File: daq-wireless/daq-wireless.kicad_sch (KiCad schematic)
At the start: 34 parts, among them J1 5223004-2, J2 Micro_SD_Card, J3 USB_C_Receptacle_USB2.0, Q1 MMBT3904, Q2 MMBT3904, SW1 RESET, U1 ESP32-WROOM-32, U2 AMS1117, U3 FT231XS, U5 Ebyte_E01-ML01SP4

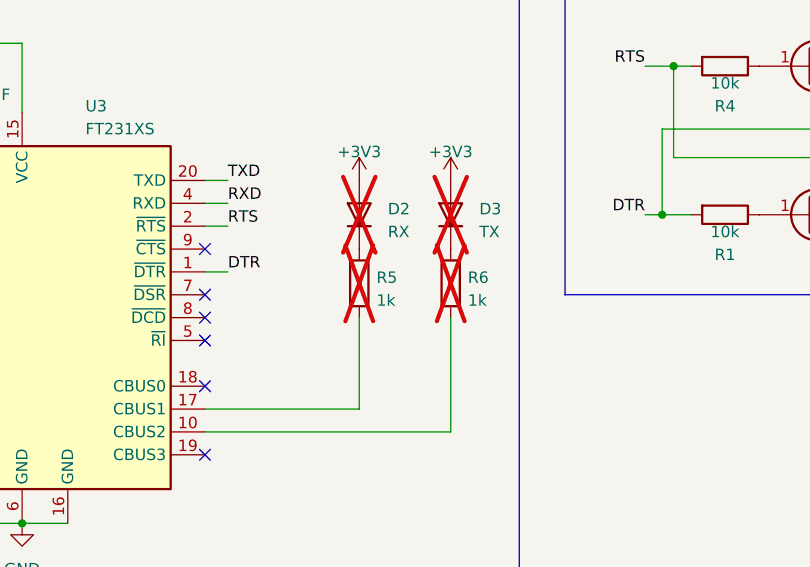
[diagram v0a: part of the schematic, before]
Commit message: BOM
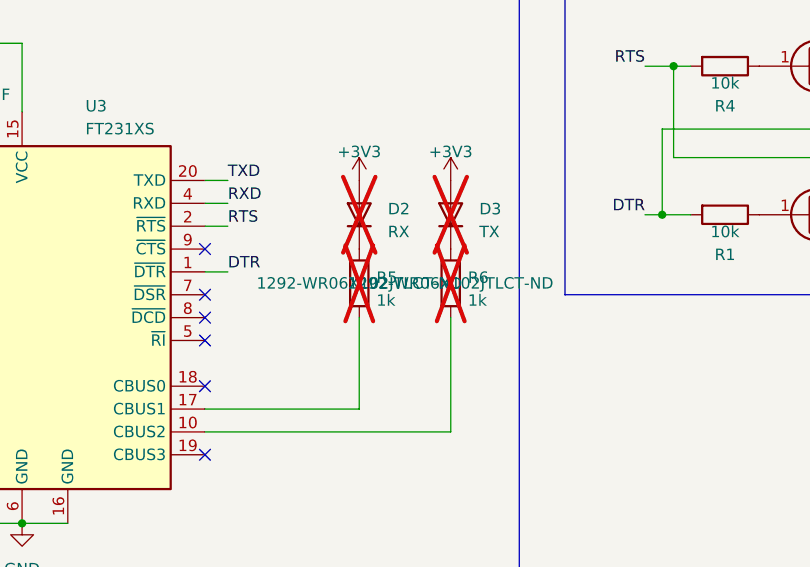
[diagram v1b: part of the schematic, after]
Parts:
- C1, C10, C3, C7, C9: DPN (none) -> 1276-1043-1-ND
- C10: footprint Capacitor_SMD:C_0402_1005Metric -> Capacitor_SMD:C_0603_1608Metric; DPN (none) -> 1276-1102-1-ND
- C2, C6, C8: DPN (none) -> 1276-1102-1-ND
- C4, C5: DPN (none) -> 1276-6460-1-ND
- C8: DPN (none) -> 1276-1119-1-ND
- R1, R4, R7, R8, R9: DPN (none) -> 1292-WR06X103JTLCT-ND
- R2, R3: DPN (none) -> RMCF0603JT5K10CT-ND
- R5, R6: DPN (none) -> 1292-WR06X102JTLCT-ND
- SW1: DPN (none) -> 2223-TS02-66-43-BK-160-LCR-D-ND
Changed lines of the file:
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@@
+      (effects (font (size 1.27 1.27)) hide)
+    )
+    (property "DPN" "1276-6460-1-ND" (at 244.475 142.24 0)
       (effects (font (size 1.27 1.27)) hide)
     )
@@
       (effects (font (size 1.27 1.27)) hide)
     )
+    (property "DPN" "1276-1102-1-ND" (at 83.185 136.525 0)
+      (effects (font (size 1.27 1.27)) hide)
+    )
     (pin "1")
     (pin "2")
@@
     )
     (property "Datasheet" "~" (at 257.81 74.93 0)
+      (effects (font (size 1.27 1.27)) hide)
+    )
+    (property "DPN" "1292-WR06X103JTLCT-ND" (at 257.81 74.93 0)
       (effects (font (size 1.27 1.27)) hide)
     )
@@
       (effects (font (size 1.27 1.27)) (justify left))
     )
-    (property "Footprint" "Capacitor_SMD:C_0402_1005Metric" (at 107.6452 54.61 0)
+    (property "Footprint" "Capacitor_SMD:C_0603_1608Metric" (at 107.6452 54.61 0)
       (effects (font (size 1.27 1.27)) hide)
     )
     (property "Datasheet" "~" (at 106.68 50.8 0)
+      (effects (font (size 1.27 1.27)) hide)
+    )
+    (property "DPN" "1276-1102-1-ND" (at 106.68 50.8 0)
       (effects (font (size 1.27 1.27)) hide)
     )
@@
       (effects (font (size 1.27 1.27)) hide)
     )
-    (property "DPN" "" (at 252.73 103.505 0)
+    (property "DPN" "1292-WR06X103JTLCT-ND" (at 252.73 103.505 0)
       (effects (font (size 1.27 1.27)) hide)
     )
@@
       (effects (font (size 1.27 1.27)) hide)
     )
+    (property "DPN" "1276-1119-1-ND" (at 227.33 81.915 0)
+      (effects (font (size 1.27 1.27)) hide)
+    )
     (pin "1")
     (pin "2")
@@
       (effects (font (size 1.27 1.27)) hide)
     )
-    (property "DPN" "" (at 140.335 159.385 0)
+    (property "DPN" "1292-WR06X102JTLCT-ND" (at 140.335 159.385 0)
       (effects (font (size 1.27 1.27)))
     )
@@
       (effects (font (size 1.27 1.27)) hide)
     )
+    (property "DPN" "1276-6460-1-ND" (at 219.075 142.24 0)
+      (effects (font (size 1.27 1.27)) hide)
+    )
     (pin "1")
     (pin "2")
@@
     )
     (property "Datasheet" "~" (at 85.09 182.245 0)
+      (effects (font (size 1.27 1.27)) hide)
+    )
+    (property "DPN" "1276-1043-1-ND" (at 85.09 182.245 0)
       (effects (font (size 1.27 1.27)) hide)
     )
@@
       (effects (font (size 1.27 1.27)) hide)
     )
+    (property "DPN" "RMCF0603JT5K10CT-ND" (at 55.88 151.13 0)
+      (effects (font (size 1.27 1.27)) hide)
+    )
     (pin "1")
     (pin "2")
@@
     )
     (property "Datasheet" "~" (at 240.665 42.545 0)
+      (effects (font (size 1.27 1.27)) hide)
+    )
+    (property "DPN" "1276-1043-1-ND" (at 240.665 42.545 0)
       (effects (font (size 1.27 1.27)) hide)
     )
@@
       (effects (font (size 1.27 1.27)) hide)
     )
+    (property "DPN" "1276-1043-1-ND" (at 215.265 81.915 0)
+      (effects (font (size 1.27 1.27)) hide)
+    )
     (pin "1")
     (pin "2")
@@
       (effects (font (size 1.27 1.27)) hide)
     )
+    (property "DPN" "1292-WR06X103JTLCT-ND" (at 180.975 135.255 0)
+      (effects (font (size 1.27 1.27)) hide)
+    )
     (pin "1")
     (pin "2")
@@
     )
     (property "Datasheet" "~" (at 125.095 36.195 0)
+      (effects (font (size 1.27 1.27)) hide)
+    )
+    (property "DPN" "1276-1043-1-ND" (at 125.095 36.195 0)
       (effects (font (size 1.27 1.27)) hide)
     )
@@
     )
     (property "Datasheet" "~" (at 113.665 36.195 0)
+      (effects (font (size 1.27 1.27)) hide)
+    )
+    (property "DPN" "1276-1102-1-ND" (at 113.665 36.195 0)
       (effects (font (size 1.27 1.27)) hide)
     )
@@
       (effects (font (size 1.27 1.27)) hide)
     )
+    (property "DPN" "2223-TS02-66-43-BK-160-LCR-D-ND" (at 250.19 80.645 0)
+      (effects (font (size 1.27 1.27)) hide)
+    )
     (pin "1")
     (pin "2")
@@
       (effects (font (size 1.27 1.27)) hide)
     )
-    (property "DPN" "" (at 252.73 111.125 0)
+    (property "DPN" "1292-WR06X103JTLCT-ND" (at 252.73 111.125 0)
       (effects (font (size 1.27 1.27)) hide)
     )
@@
     )
     (property "Datasheet" "~" (at 180.975 151.765 0)
+      (effects (font (size 1.27 1.27)) hide)
+    )
+    (property "DPN" "1292-WR06X103JTLCT-ND" (at 180.975 151.765 0)
       (effects (font (size 1.27 1.27)) hide)
     )
@@
       (effects (font (size 1.27 1.27)) hide)
     )
-    (property "DPN" "" (at 150.495 159.385 0)
+    (property "DPN" "1292-WR06X102JTLCT-ND" (at 150.495 159.385 0)
       (effects (font (size 1.27 1.27)))
     )
@@
     )
     (property "Datasheet" "~" (at 94.615 136.525 0)
+      (effects (font (size 1.27 1.27)) hide)
+    )
+    (property "DPN" "1276-1043-1-ND" (at 94.615 136.525 0)
       (effects (font (size 1.27 1.27)) hide)
     )
@@
     )
     (property "Datasheet" "~" (at 252.73 42.545 0)
+      (effects (font (size 1.27 1.27)) hide)
+    )
+    (property "DPN" "1276-1102-1-ND" (at 252.73 42.545 0)
       (effects (font (size 1.27 1.27)) hide)
     )
@@
       (effects (font (size 1.27 1.27)) hide)
     )
+    (property "DPN" "RMCF0603JT5K10CT-ND" (at 55.88 153.67 0)
+      (effects (font (size 1.27 1.27)) hide)
+    )
